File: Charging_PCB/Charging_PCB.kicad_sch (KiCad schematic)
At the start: 15 parts, among them K3 Relay_SPDT_Omron_G2RL-1, K4 Relay_SPDT_Omron_G2RL-1, Q3 Q_PMOS_GSD, Q4 Q_PMOS_GSD, U112 641964-1, U113 641964-1, U114 641964-1

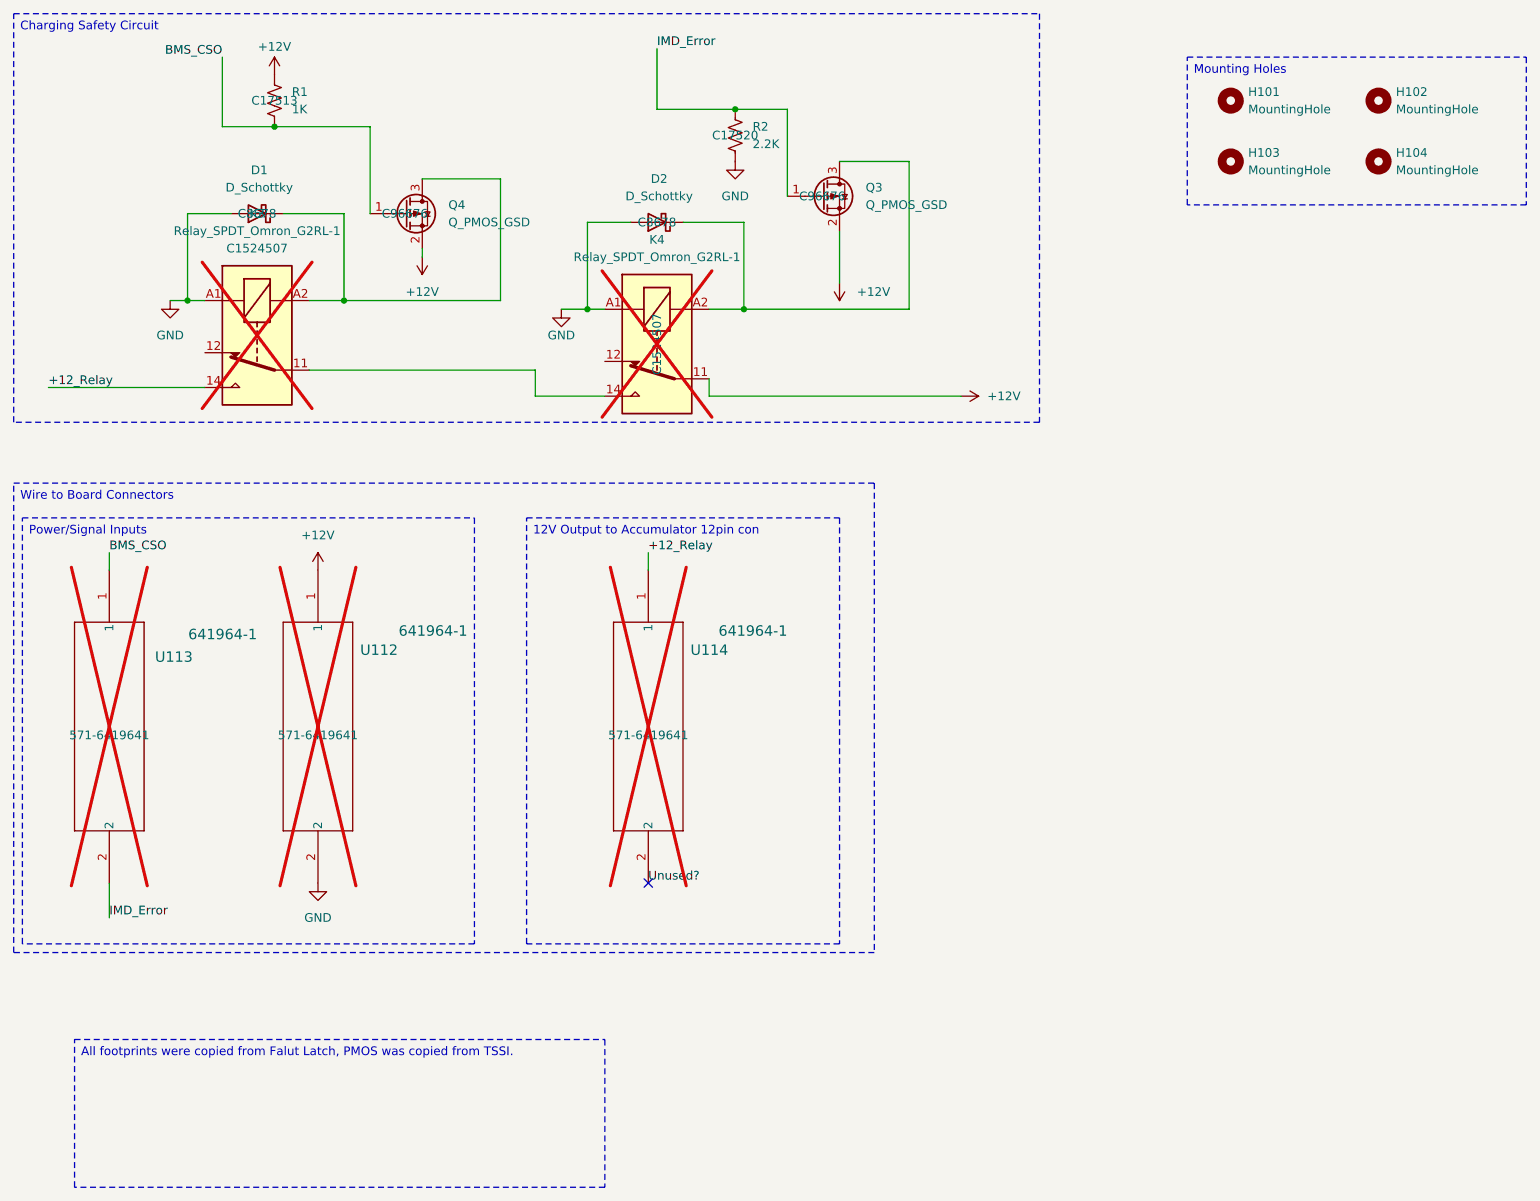
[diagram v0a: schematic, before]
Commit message: CHARGE READY
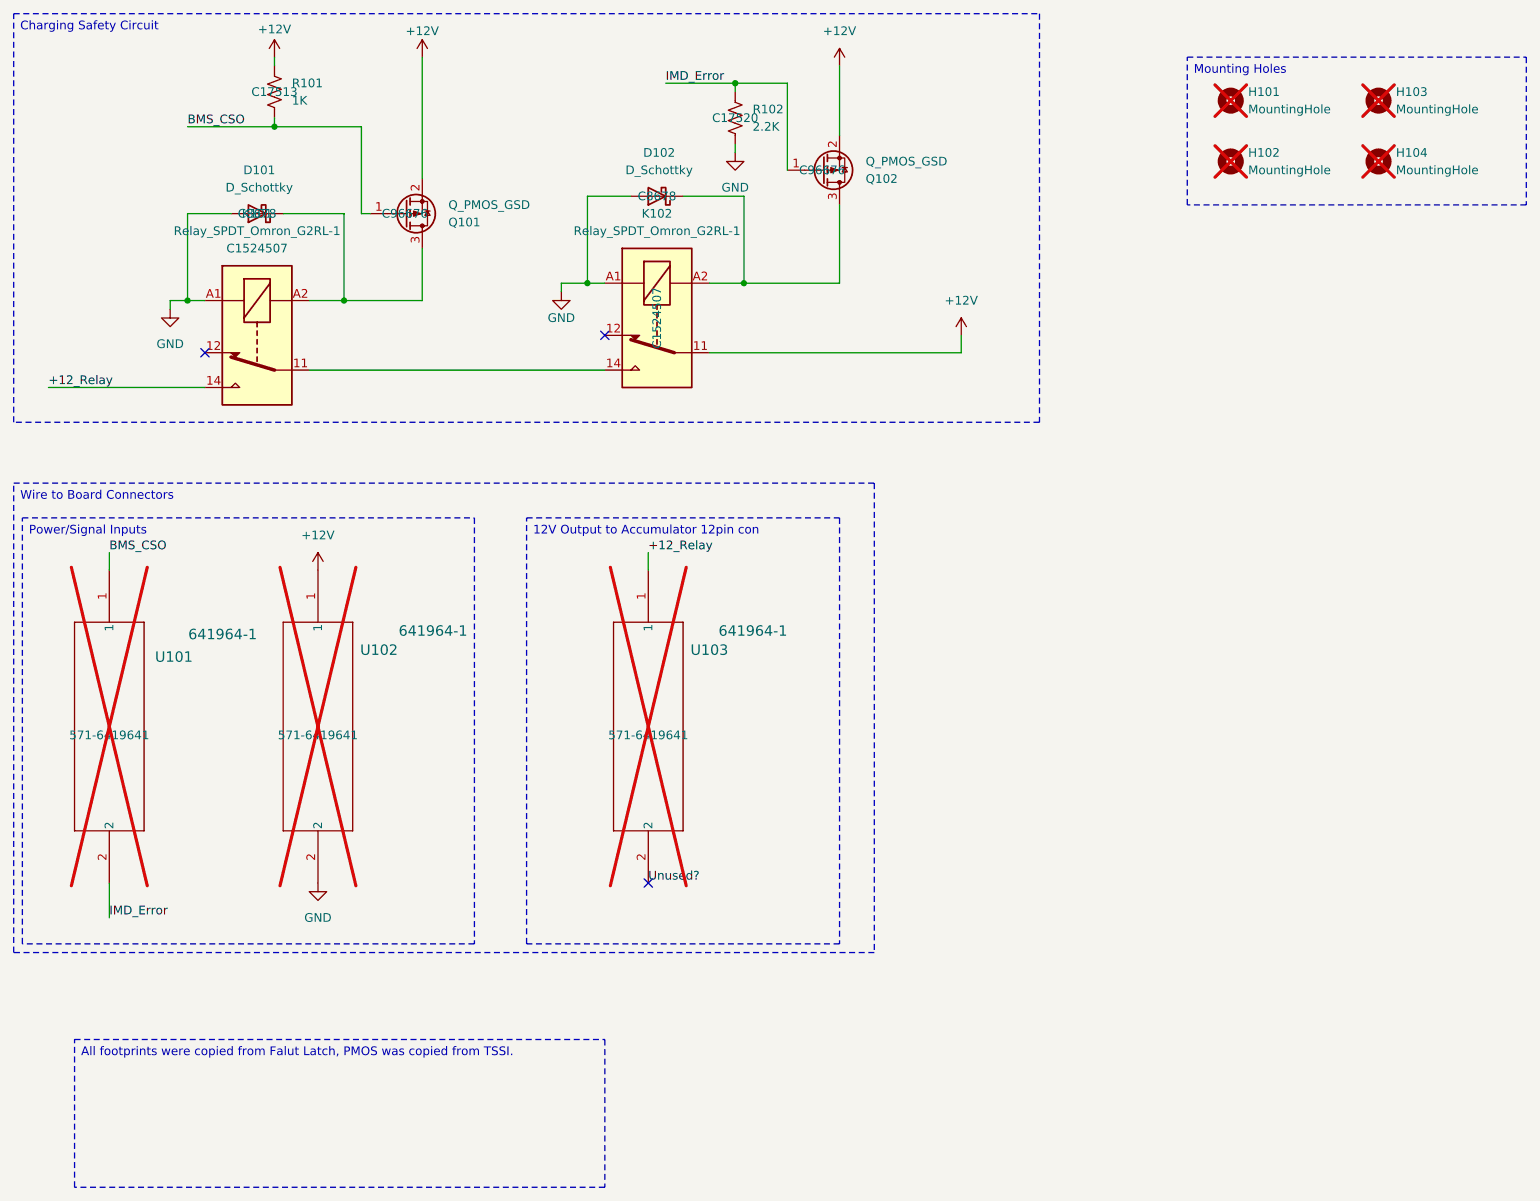
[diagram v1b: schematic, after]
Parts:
- H101, H104: now not fitted
- H102: renamed from H103; now not fitted
- H103: renamed from H102; now not fitted
- K101: renamed from K3; now fitted; now in the parts list
- K102: renamed from K4; now fitted; now in the parts list
- renumbered D1 to D101, D2 to D102, Q4 to Q101, Q3 to Q102, R1 to R101, R2 to R102, U113 to U101, U112 to U102, U114 to U103
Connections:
- no-connect marks 1 -> 3
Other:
- moved on the sheet: D102, Q102, R101, R102
